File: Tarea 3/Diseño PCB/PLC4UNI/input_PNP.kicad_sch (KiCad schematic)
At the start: 0 parts

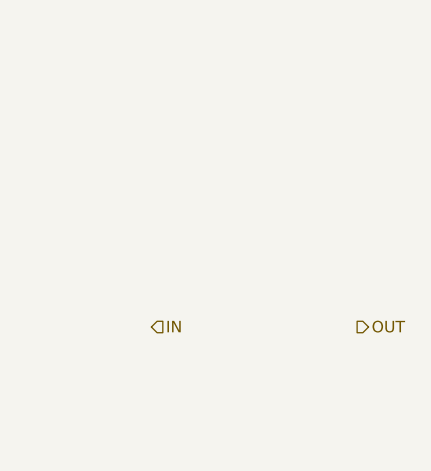
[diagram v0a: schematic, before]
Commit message: Tarea 3
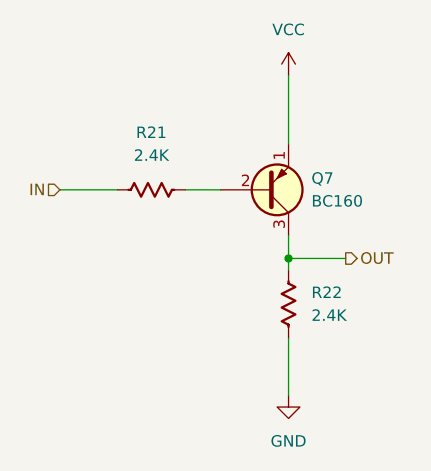
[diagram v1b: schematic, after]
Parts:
- added Q7: BC160, PCM_Package_TO_SOT_THT_AKL:TO-39-3_EBC, symbol PCM_Transistor_BJT_AKL:BC160
- added R21, R22: 2.4K, PCM_Resistor_SMD_AKL:R_0603_1608Metric, symbol PCM_Resistor_US_AKL:R_0603
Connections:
- net IN: now also R21.1
- net OUT: now also Q7.3 (C), R22.2
- new net: Q7.2 (B), R21.2
- new net GND: R22.1
- new net VCC: Q7.1 (E)

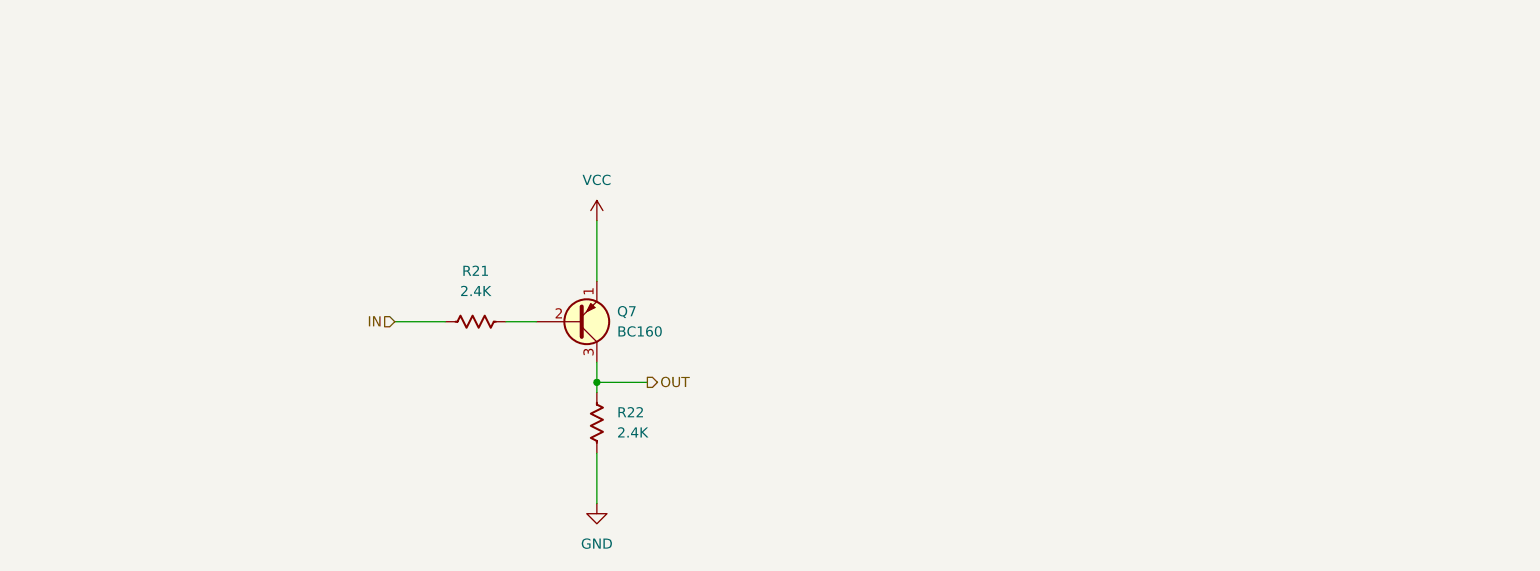
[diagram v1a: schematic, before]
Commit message: Tarea 3
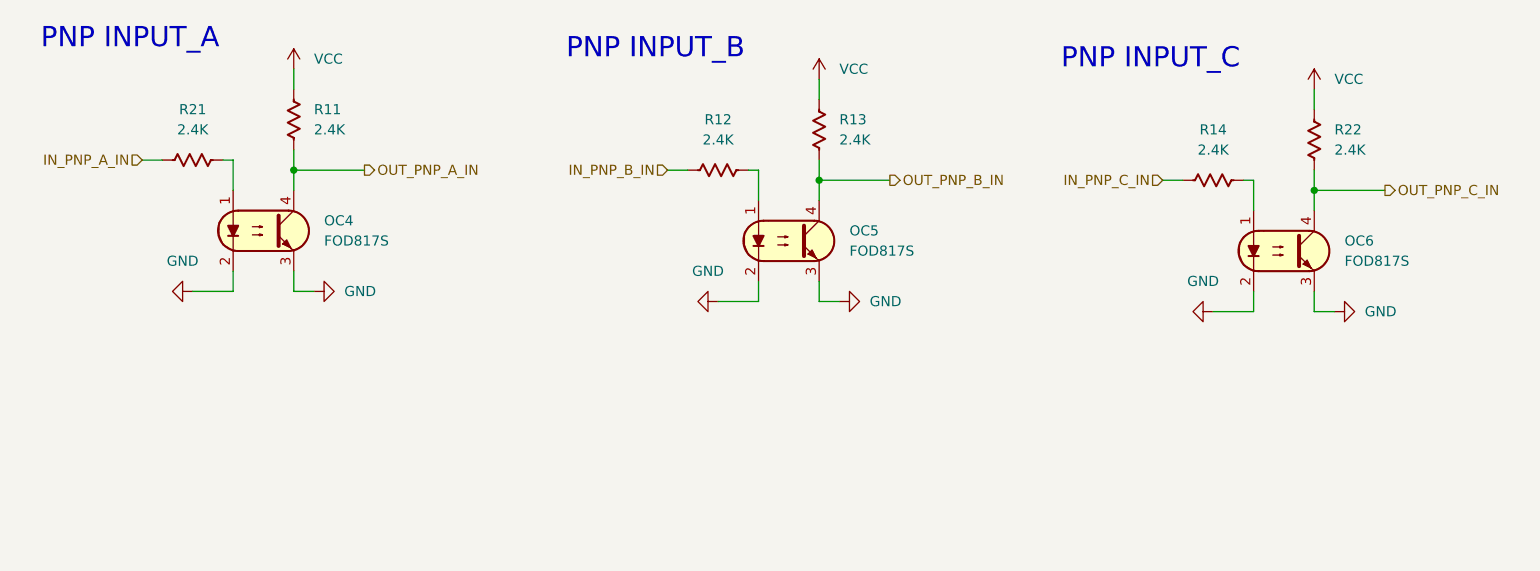
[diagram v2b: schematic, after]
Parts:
- removed Q7: BC160, PCM_Package_TO_SOT_THT_AKL:TO-39-3_EBC, symbol PCM_Transistor_BJT_AKL:BC160
- added OC4, OC5, OC6: FOD817S, PCM_Package_DIP_AKL:SMDIP-4_W9.53mm, symbol PCM_Optocoupler_AKL:FOD817S
- added R11, R12, R13, R14: 2.4K, PCM_Resistor_SMD_AKL:R_0603_1608Metric, symbol PCM_Resistor_US_AKL:R_0603
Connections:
- net OUT is gone; now on net VCC: R22.2
- net GND: now also OC4.2, OC4.3, OC5.2, OC5.3, OC6.2, OC6.3; no longer R22.1
- net VCC: now also R11.2, R13.2
- net at R21.2: now also OC4.1
- net IN renamed IN_PNP_A_IN
- new net: OC5.1, R12.2
- new net: OC6.1, R14.2
- new net IN_PNP_B_IN: R12.1
- new net IN_PNP_C_IN: R14.1
- new net OUT_PNP_A_IN: OC4.4, R11.1
- new net OUT_PNP_B_IN: OC5.4, R13.1
- new net OUT_PNP_C_IN: OC6.4, R22.1
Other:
- note added: "PNP INPUT_A"
- note added: "PNP INPUT_B"
- note added: "PNP INPUT_C"
- moved on the sheet: R21
